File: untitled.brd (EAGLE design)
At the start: 59.7 x 68.2 mm, 10 parts

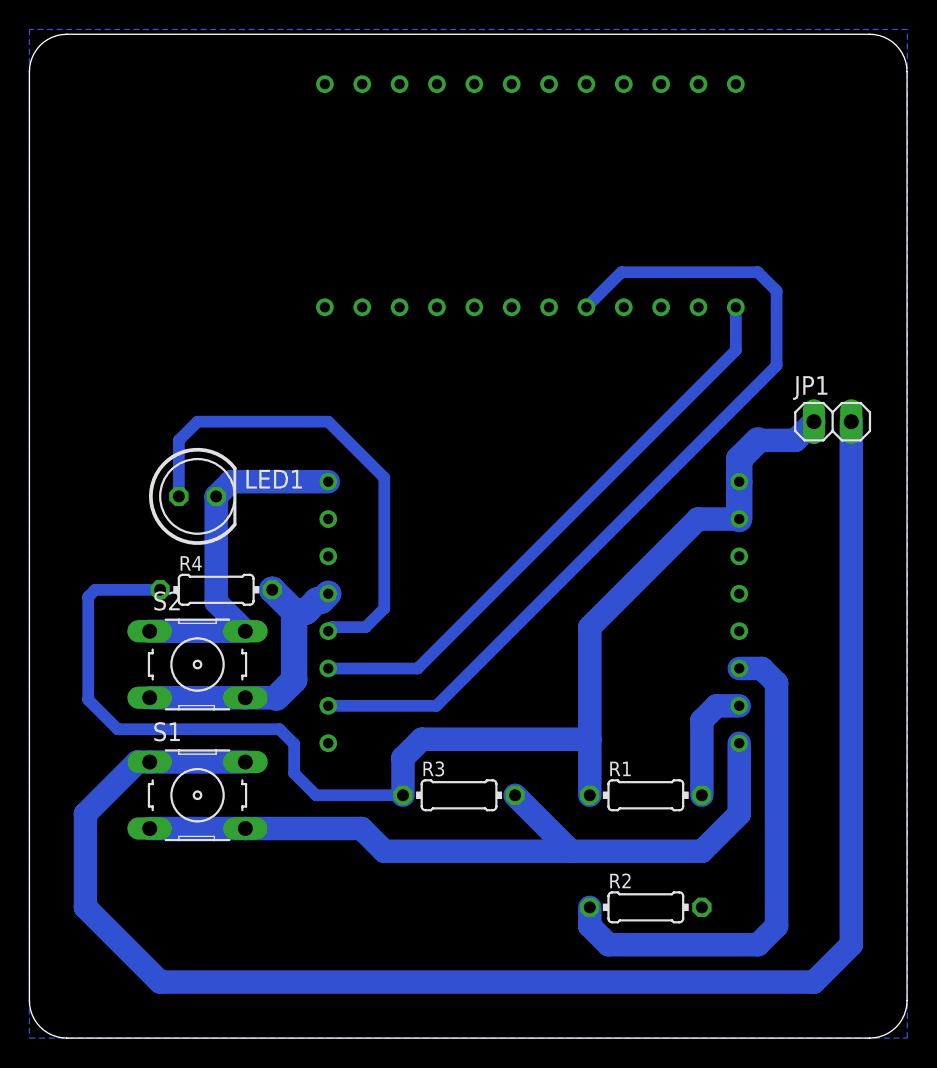
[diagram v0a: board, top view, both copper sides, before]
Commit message: Maybe Complete
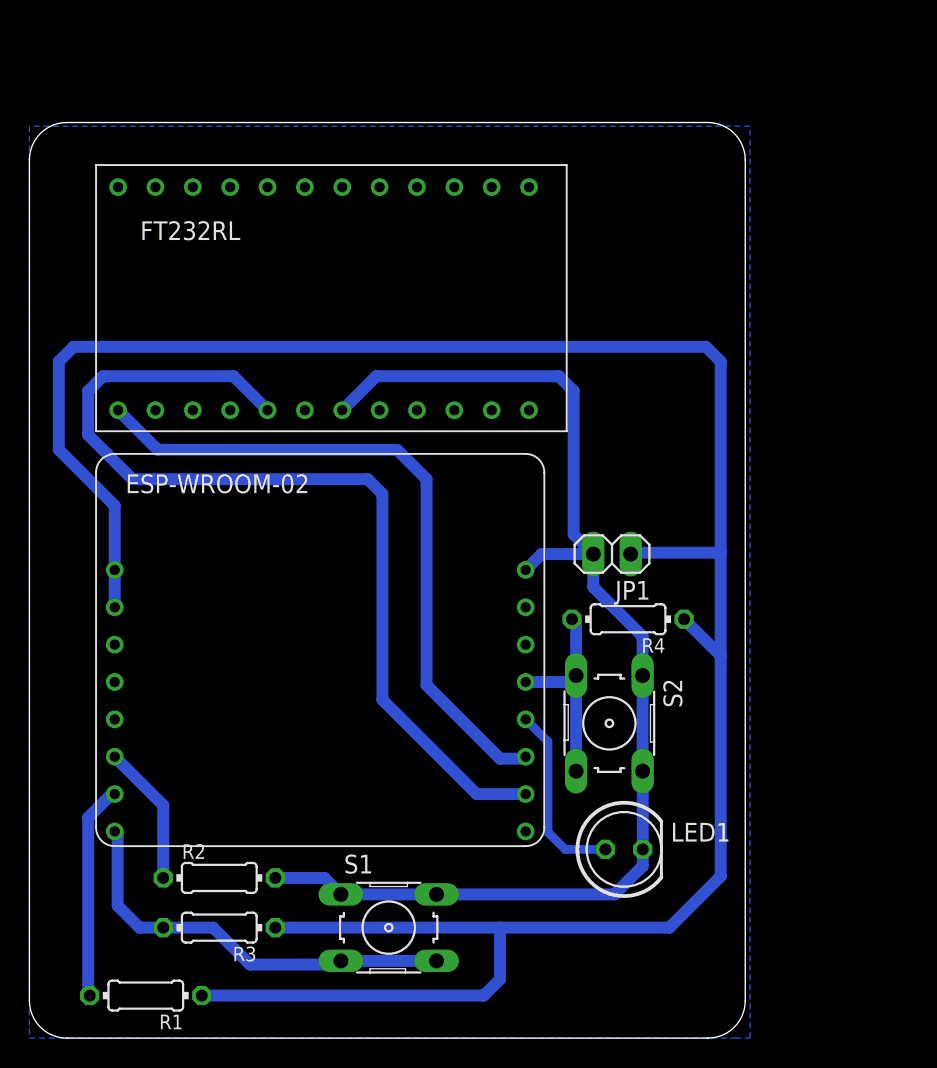
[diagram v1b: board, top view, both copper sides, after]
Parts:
- moved FT232RL1 45.5 mm to (4.53, 41.3), flipped to the top
- moved ESP-WROOM-1 45.4 mm to (4.53, 13.1), flipped to the top
- moved LED1 37.6 mm to (40.4, 12.8)
- moved R1 36.6 mm to (7.91, 2.89), turned to 180 degrees
- moved R2 29.1 mm to (12.9, 10.9)
- moved S2 28.3 mm to (39.4, 21.4), turned to 270 degrees
- moved R4 28.1 mm to (40.7, 28.5), turned to 180 degrees
- moved R3 18.6 mm to (12.9, 7.51), turned to 180 degrees
- moved JP1 17.5 mm to (39.6, 32.9), turned to 180 degrees
- moved S1 15.8 mm to (24.4, 7.51)
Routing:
- net 3V3: track 88.0 -> 164.8 mm
- net GND: track 134.0 -> 82.6 mm
- net IO15: track 34.5 -> 9.61 mm
- net IO0: track 52.0 -> 28.6 mm
- net IO5: track 33.2 -> 12.7 mm
- net IO2: track 8.03 -> 14.6 mm
- net TXD: track 39.6 -> 45.8 mm
- net RST: track 19.9 -> 14.1 mm
- net RXD: track 59.6 -> 64.6 mm
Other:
- board size 59.7 x 68.2 mm -> 48.7 x 62.2 mm
